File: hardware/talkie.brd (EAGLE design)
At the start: 72 x 26 mm, 81 parts, among them X1 12MHz

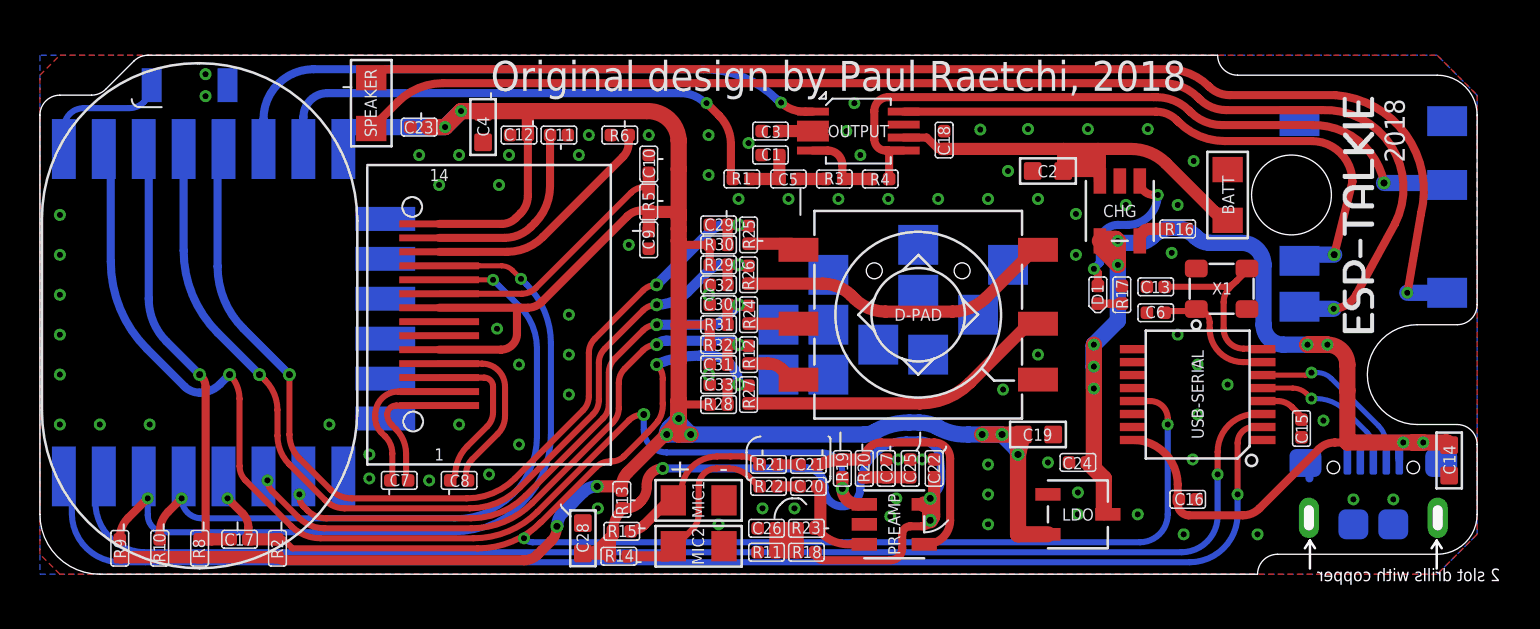
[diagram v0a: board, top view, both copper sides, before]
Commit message: Latest files (also sent to pcbway and jlcpcb)
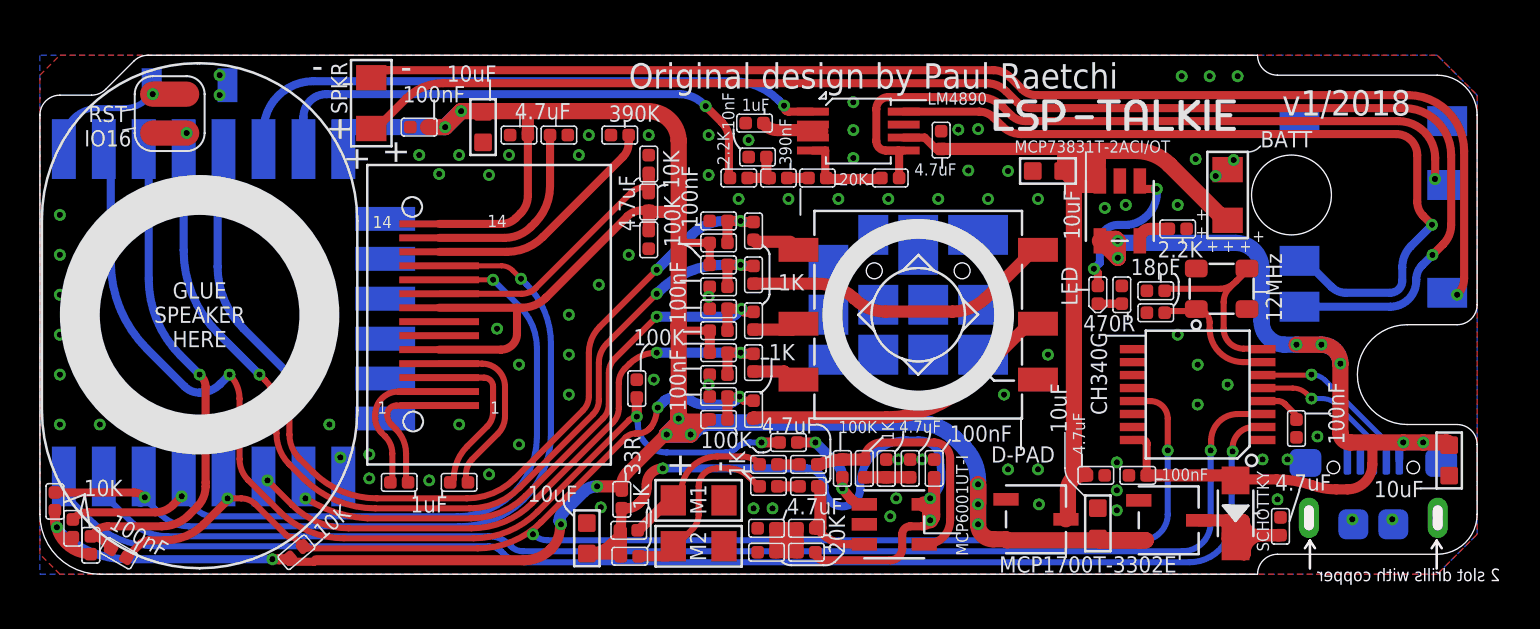
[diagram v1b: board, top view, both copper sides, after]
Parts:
- removed LDO: MCP1700T, parts:SOT-23-3
- added C34: 4.7uF, Seeed-OPL-Capacitor:C0402
- added D2: SCHOTTKY, Seeed-OPL-Diode:SOD-123
- added LDO1: MCP1700T, parts:SOT-23-3
- added LDO2: MCP1700T-3302E, parts:SOT-23-3
- added R33, R7: 100K, Seeed-OPL-Resistor:R0402
- CPU: value (none) -> ESP-12E
- R10, R2, R5, R8, R9: value 10k -> 10K
- R6: value 390k -> 390K
- SPEAKER: value SPEAKER -> SPKR
- moved C24 10.6 mm to (62.1, 2.40), turned to 180 degrees
- moved C17 6.09 mm to (3.95, 1.05), turned to 60 degrees
- moved R8 5.45 mm to (2.55, 1.45)
- moved C19 5.37 mm to (53.0, 2.55), turned to 180 degrees
- moved R10 4.46 mm to (1.65, 2.30)
- moved R9 4.01 mm to (0.75, 3.65)
- moved C16 2.77 mm to (55.0, 4.95), turned to 90 degrees
- moved R2 0.97 mm to (12.8, 1.10), turned to 310 degrees
- moved C3 0.89 mm to (35.8, 22.6)
- moved R3 0.85 mm to (39.0, 19.9)
- moved R27 0.79 mm to (35.8, 8.25)
- moved R28 0.75 mm to (34.0, 7.75)
- moved C1 0.66 mm to (36.0, 20.9)
- moved C33 0.60 mm to (34.0, 8.90)
- moved R14 0.55 mm to (29.6, 0.90)
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- renumbered MIC1 to M1, MIC2 to M2, RST to RESET, U2 to CPU
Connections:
- new net OUT: PREAMP.1, R19.2, R7.2
- new net VIN: C24.1, D2.-, LDO2.3
- net 3V3: now also LDO1.2, LDO2.2; no longer LDO.2
- net ADC: now also R33.2, R7.1; no longer PREAMP.1, R19.2
- net GND: now also C34.2, LDO1.1, LDO2.1, R33.1; no longer LDO.1
- net VBAT: now also C34.1, LDO1.3
- net VBUS: now also D2.+; no longer C24.1, LDO.3
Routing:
- net VBUS: track 85.5 -> 48.0 mm, vias 9 -> 7
- net VBAT: track 24.8 -> 48.4 mm
- net 3V3: track 135.7 -> 156.0 mm, vias 10 -> 12
- net VIN: track 0.00 -> 11.5 mm
- net R: track 29.3 -> 39.9 mm
- net SPK+: track 62.5 -> 69.6 mm
- net OUT: track 0.00 -> 5.66 mm, vias 0 -> 2
- net ADC: track 58.9 -> 53.3 mm
- net SCL: track 34.7 -> 38.7 mm
- net EN: track 22.2 -> 25.9 mm
- net BTN4: track 48.8 -> 52.4 mm, vias 3 -> 4
- net BOOT: track 77.4 -> 79.8 mm
- net SDA: track 40.2 -> 42.4 mm
- net SPK-: track 62.0 -> 64.2 mm
- net RST: track 6.50 -> 8.23 mm, vias 0 -> 1
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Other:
- outline, holes or cut-outs redrawn
- board text added: "BATTERY"
- board text added: "GLUE SPEAKER HERE"
- board text added: "JACK"
- board text added: "Original design by Paul Raetchi"
- board text added: "RST IO16"
- board text added: "v1/2018"
- board text removed: "Original design by Paul Raetchi, 2018"
